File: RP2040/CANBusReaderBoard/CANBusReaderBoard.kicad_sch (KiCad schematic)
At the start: 13 parts, among them J0 RJ45, J1 RJ45, J2 RJ45, J3 RJ45, U1 MCP2515-xSO, U1 RP2040, Y1 Crystal

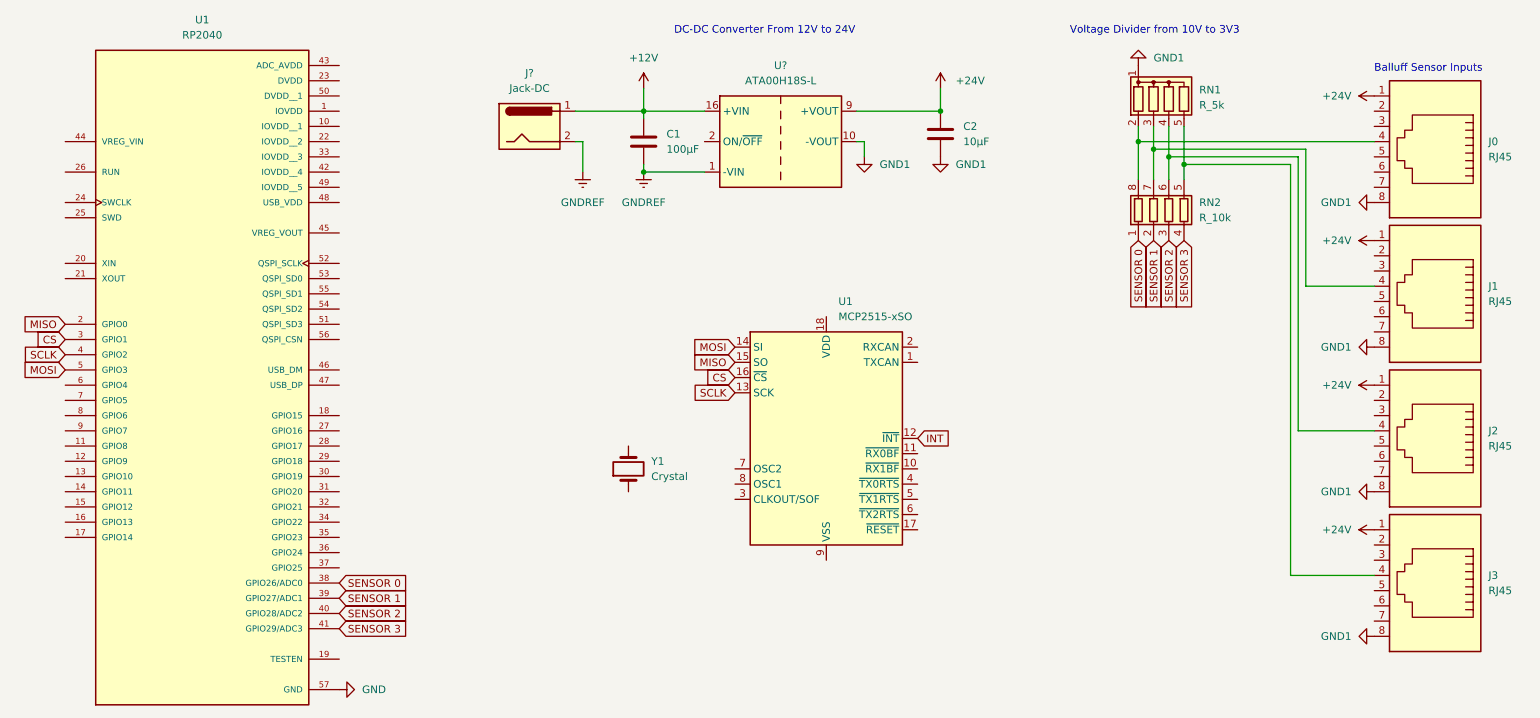
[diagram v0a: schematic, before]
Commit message: Components all added, need to figure out RP2040 Powering and supplemental components.
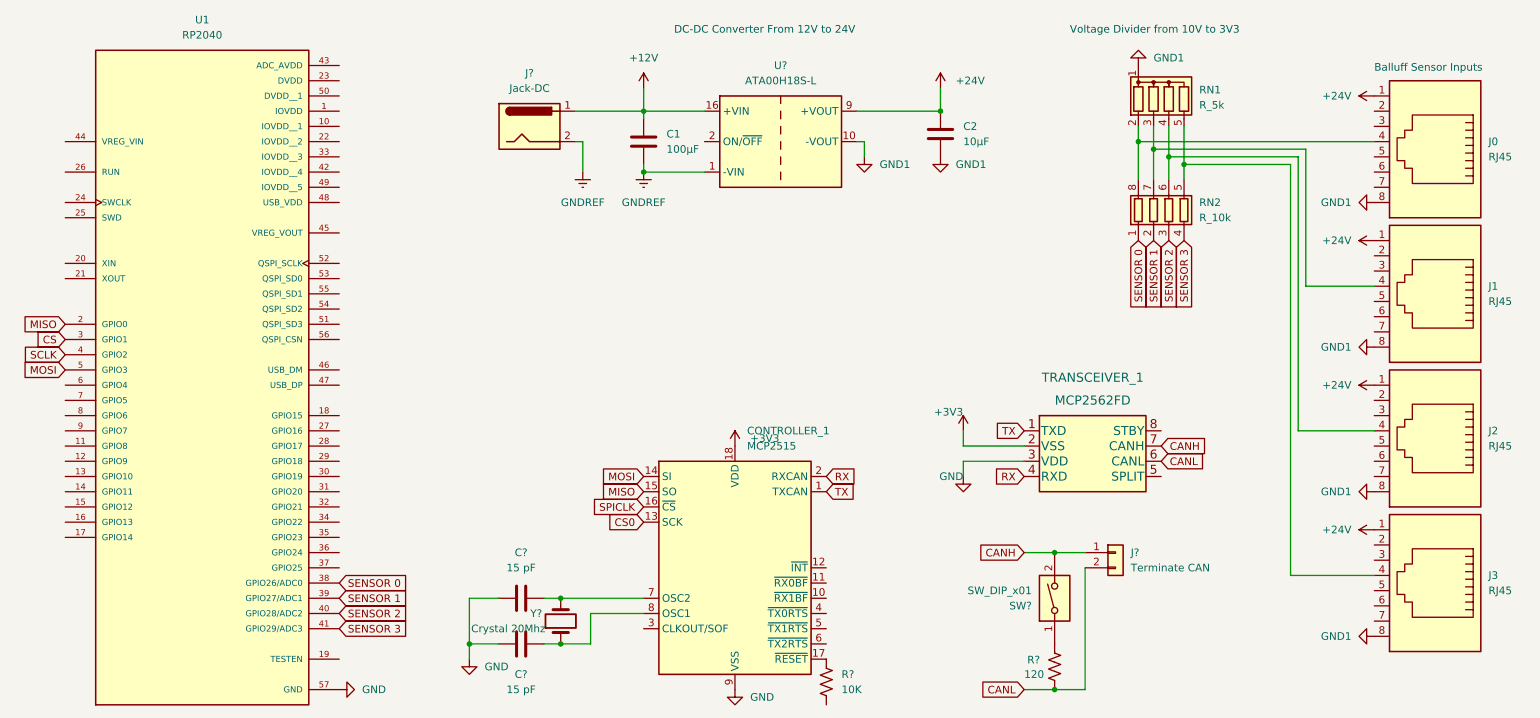
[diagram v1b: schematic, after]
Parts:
- removed U1: MCP2515-xSO, Package_SO:SOIC-18W_7.5x11.6mm_P1.27mm, symbol Interface_CAN_LIN:MCP2515-xSO
- removed Y1: Crystal, symbol Device:Crystal
- added C? (x2): 15 pF, Capacitor_THT:C_Axial_L3.8mm_D2.6mm_P7.50mm_Horizontal, symbol Device:C
- added CONTROLLER_1: MCP2515, MCP2515:MCP2515-E&slash_P, symbol Interface_CAN_LIN:MCP2515-xSO
- added J?: Terminate CAN, TerminalBlock_Phoenix:TerminalBlock_Phoenix_MKDS-3-2-5.08_1x02_P5.08mm_Horizontal, symbol Connector_Generic:Conn_01x02
- added R?: 120, Resistor_THT:R_Axial_DIN0204_L3.6mm_D1.6mm_P5.08mm_Horizontal, symbol Device:R_US
- added R?: 10K, Resistor_THT:R_Axial_DIN0204_L3.6mm_D1.6mm_P5.08mm_Horizontal, symbol Device:R_US
- added SW?: SW_DIP_x01, symbol Switch:SW_DIP_x01
- added TRANSCEIVER_1: MCP2562FD, MCP2562FD:MCP2562FD-H&slash_P, symbol MCP2562FD:MCP2562FD-H/P
- added Y?: Crystal 20Mhz, symbol Device:Crystal
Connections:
- net GND: now also C?.1, C?.1, CONTROLLER_1.9 (VSS), TRANSCEIVER_1.3 (VDD)
- net MISO: now also CONTROLLER_1.15 (SO)
- net MOSI: now also CONTROLLER_1.14 (SI)
- new net: R?.1, SW?.1
- new net: C?.2, CONTROLLER_1.8 (OSC1), Y?.1
- new net: C?.2, CONTROLLER_1.7 (OSC2), Y?.2
- new net: CONTROLLER_1.17 (~{RESET}), R?.1
- new net +3V3: CONTROLLER_1.18 (VDD), TRANSCEIVER_1.2 (VSS)
- new net CANH: J?.1 (Pin_1), SW?.2, TRANSCEIVER_1.7 (CANH)
- new net CANL: J?.2 (Pin_2), R?.2, TRANSCEIVER_1.6 (CANL)
- new net CS0: CONTROLLER_1.13 (SCK)
- new net RX: CONTROLLER_1.2 (RXCAN), TRANSCEIVER_1.4 (RXD)
- new net SPICLK: CONTROLLER_1.16 (~{CS})
- new net TX: CONTROLLER_1.1 (TXCAN), TRANSCEIVER_1.1 (TXD)
